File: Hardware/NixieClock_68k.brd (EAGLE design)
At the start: 100 x 100 mm, 56 parts, among them IC1 68008, IC10 7805, IC11 MIC803, IC12 74HC08N, IC2 AS6C1008, IC3 39SF020, IC4 DS1244Y, IC5 68681, IC6 74HC30N, IC7 74HC04N, IC8 74HC138N, IC9 74HC266N, Q1 4MHz, Q2 3.6864MHz

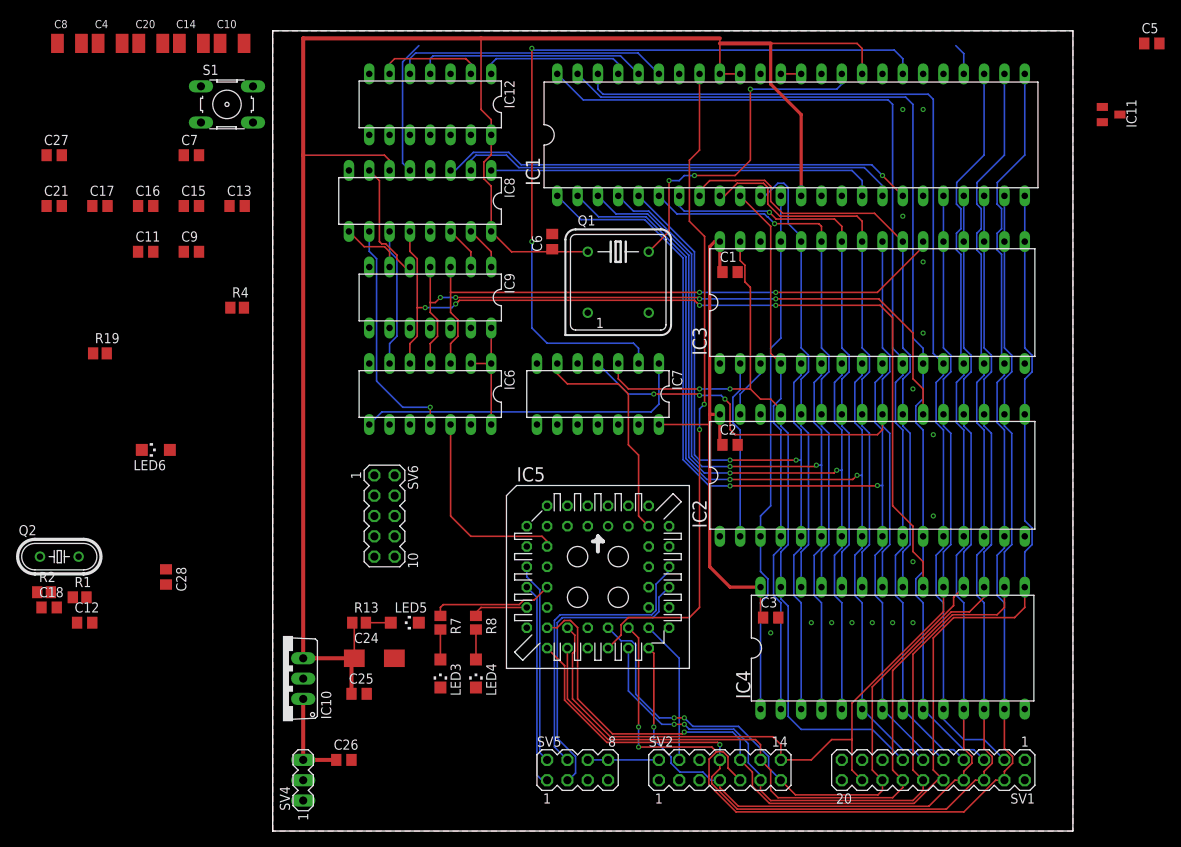
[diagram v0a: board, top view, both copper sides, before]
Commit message: finished routing main board
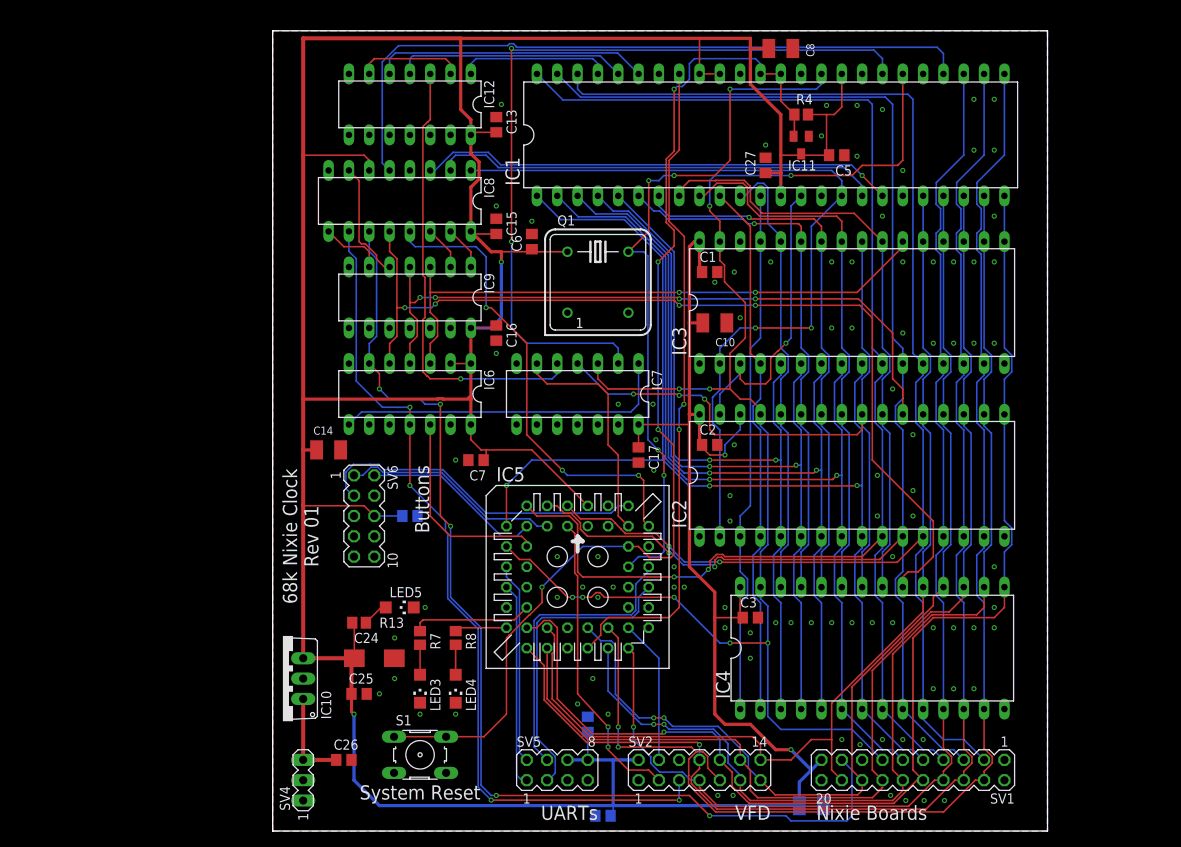
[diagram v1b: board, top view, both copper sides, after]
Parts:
- removed C12, C18: 27pF, rcl:C0805
- removed C20: 10µF, rcl:SMC_B
- removed C21: 100nF, rcl:C0805
- removed LED6: (no value), led:CHIPLED_1206
- removed Q2: 3.6864MHz, crystal:HC49/S
- removed R1, R2: 100R, rcl:R2012
- removed R19: 3k, rcl:R2012
- Q1: value 4MHz -> 3.6864MHz
- moved C4 129.4 mm to (67.3, 3.17), flipped to the bottom, turned to 180 degrees
- moved C27 88.9 mm to (61.6, 83.2), turned to 90 degrees
- moved C8 88.9 mm to (63.5, 97.8)
- moved C9 87.3 mm to (41.3, 1.91), flipped to the bottom
- moved S1 84.8 mm to (18.4, 9.53)
- moved C11 80.9 mm to (39.4, 13.3), flipped to the bottom, turned to 90 degrees
- moved R4 74.5 mm to (66.0, 89.5)
- moved C17 74.2 mm to (45.7, 47.0), turned to 270 degrees
- moved C10 69.7 mm to (55.2, 63.5)
- moved C14 53.6 mm to (6.99, 47.6)
- moved C7 52.1 mm to (25.4, 46.4), turned to 180 degrees
- moved C16 46.6 mm to (27.9, 62.2), turned to 270 degrees
- moved C5 41.8 mm to (70.5, 84.5)
- moved IC11 38.9 mm to (66.0, 85.7), turned to 180 degrees
- moved C15 38.2 mm to (27.9, 75.6), turned to 90 degrees
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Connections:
- removed net 68681_X1: IC5.36, R2.1
- removed net 68681_X2: IC5.37, R1.2
- removed net N$1: C12.1, Q2.2, R1.1
- removed net N$2: C18.1, Q2.1, R2.2
- removed net N$6: LED6.A, R19.2
- removed net STATUS2: IC5.31
- removed net STATUS3: IC5.15, R8.1
- removed net SW3: IC5.43, SV6.4
- net !RESET: no longer LED6.C
- net +5V: no longer C20.+, C21.1, R19.1, SV1.1
- net CLK: now also IC5.36
- net GND: now also SV1.1; no longer C12.2, C18.2, C20.-, C21.2
- net STATUS0: now also IC5.17, R8.1; no longer IC5.32
- net STATUS1: now also IC5.16; no longer IC5.14
- net SW0: now also IC5.5; no longer IC5.8
- net SW1: now also IC5.8; no longer IC5.5
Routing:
- net +5V: track 337.0 -> 552.1 mm, vias 0 -> 4
- net !RESET: track 2.54 -> 139.0 mm, vias 0 -> 4
- net !NIXIE_CS: track 17.3 -> 135.1 mm, vias 0 -> 5
- net R/!W!: track 100.1 -> 184.0 mm, vias 2 -> 9
- net !VFD_CS: track 29.3 -> 106.4 mm, vias 1 -> 4
- net !AS: track 20.8 -> 88.1 mm
- net !68681_CS: track 0.00 -> 59.2 mm, vias 0 -> 3
- net N$5: track 0.00 -> 56.5 mm, vias 0 -> 1
- net A2: track 131.3 -> 185.8 mm, vias 0 -> 2
- net A1: track 131.3 -> 181.7 mm, vias 0 -> 2
- net A0: track 133.6 -> 182.3 mm, vias 0 -> 2
- net CLK: track 43.0 -> 88.7 mm, vias 3 -> 5
- net SW2: track 0.00 -> 42.1 mm
- net VFD_BUSY: track 0.00 -> 37.9 mm, vias 0 -> 2
- net A16: track 71.1 -> 103.6 mm, vias 0 -> 2
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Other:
- board size 100 x 100 mm -> 96.8 x 100 mm
- board text added: "68k Nixie Clock Rev 01"
- board text added: "Buttons"
- board text added: "Nixie Boards"
- board text added: "System Reset"
- board text added: "UARTs"
- board text added: "VFD"
